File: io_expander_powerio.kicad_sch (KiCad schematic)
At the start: 14 parts, among them Q4 AO4828, Q5 AO4828

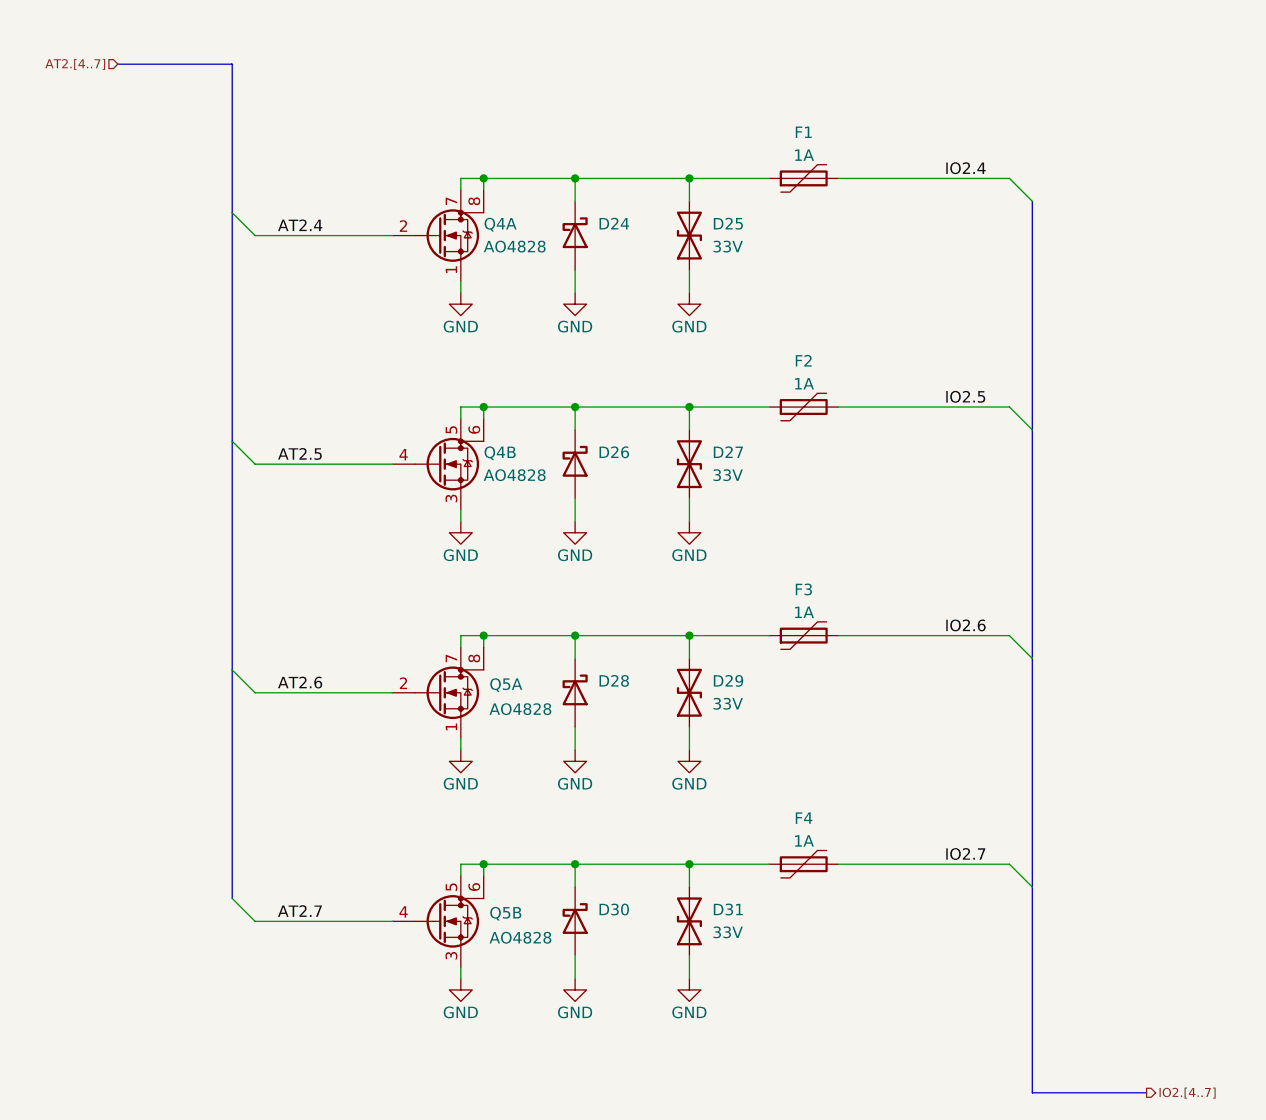
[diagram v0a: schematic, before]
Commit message: Done?
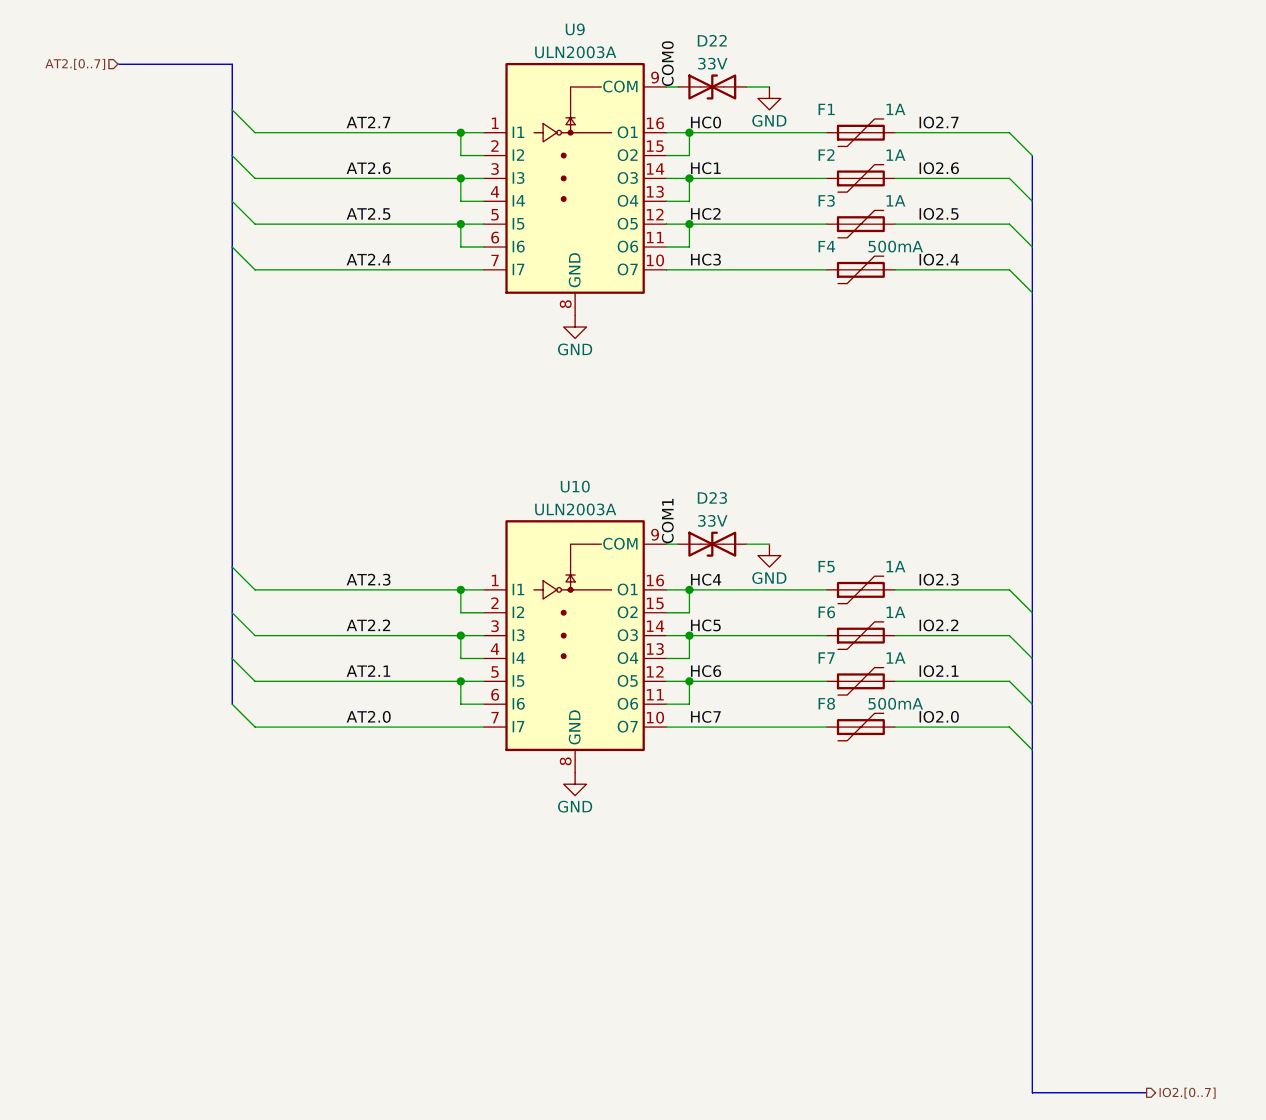
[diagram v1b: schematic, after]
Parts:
- removed D24, D26, D28, D30: D_Schottky, Diode_SMD:D_SOD-123, symbol Device:D_Schottky
- removed D25, D27, D29, D31: 33V, Diode_SMD:D_SMB, symbol Device:D_TVS
- removed Q4, Q5: AO4828, Package_SO:SOIC-8_3.9x4.9mm_P1.27mm, symbol Device:Q_Dual_NMOS_S1G1S2G2D2D2D1D1
- added D22, D23: 33V, Diode_SMD:D_SMB, symbol Device:D_TVS
- added F5, F6, F7: 1A, Fuse:Fuse_1206_3216Metric, symbol Device:Polyfuse
- added F8: 500mA, Fuse:Fuse_1206_3216Metric, symbol Device:Polyfuse
- added U10, U9: ULN2003A, Package_SO:SOIC-16_3.9x9.9mm_P1.27mm, symbol Transistor_Array:ULN2003A
- F4: value 1A -> 500mA
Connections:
- net AT2.4: now also U9.7 (I7)
- net AT2.5: now also U9.5 (I5), U9.6 (I6)
- net AT2.6: now also U9.3 (I3), U9.4 (I4)
- net AT2.7: now also U9.1 (I1), U9.2 (I2)
- net GND: now also D22.2 (A2), D23.2 (A2), U10.8 (GND), U9.8 (GND)
- net IO2.4: now also F4.2; no longer F1.2
- net IO2.5: now also F3.2; no longer F2.2
- net IO2.6: now also F2.2; no longer F3.2
- net IO2.7: now also F1.2; no longer F4.2
- net HC2: now reaches F3.1
- net HC2: now also U9.11 (O6), U9.12 (O5)
- net HC0: now reaches F1.1
- net HC0: now also U9.15 (O2), U9.16 (O1)
- net HC3: now reaches F4.1
- net HC3: now also U9.10 (O7)
- net HC1: now reaches F2.1
- net HC1: now also U9.13 (O4), U9.14 (O3)
- new net AT2.0: U10.7 (I7)
- new net AT2.1: U10.5 (I5), U10.6 (I6)
- new net AT2.2: U10.3 (I3), U10.4 (I4)
- new net AT2.3: U10.1 (I1), U10.2 (I2)
- new net COM0: D22.1 (A1), U9.9 (COM)
- new net COM1: D23.1 (A1), U10.9 (COM)
- new net HC4: F5.1, U10.15 (O2), U10.16 (O1)
- new net HC5: F6.1, U10.13 (O4), U10.14 (O3)
- new net HC6: F7.1, U10.11 (O6), U10.12 (O5)
- new net HC7: F8.1, U10.10 (O7)
- new net IO2.0: F8.2
- new net IO2.1: F7.2
- new net IO2.2: F6.2
- new net IO2.3: F5.2
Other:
- moved on the sheet: F1
